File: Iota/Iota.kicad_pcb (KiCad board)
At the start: 2 copper layers, 22.6 x 43.4 mm, 23 parts, among them J1 USB_B_Mini, J2 Conn_01x12_Male, J3 Conn_01x12_Male, J4 Conn_01x05_Male, SW1 SW_DIP_x01, U1 ATmega32U4-MU, Y1 16MHz

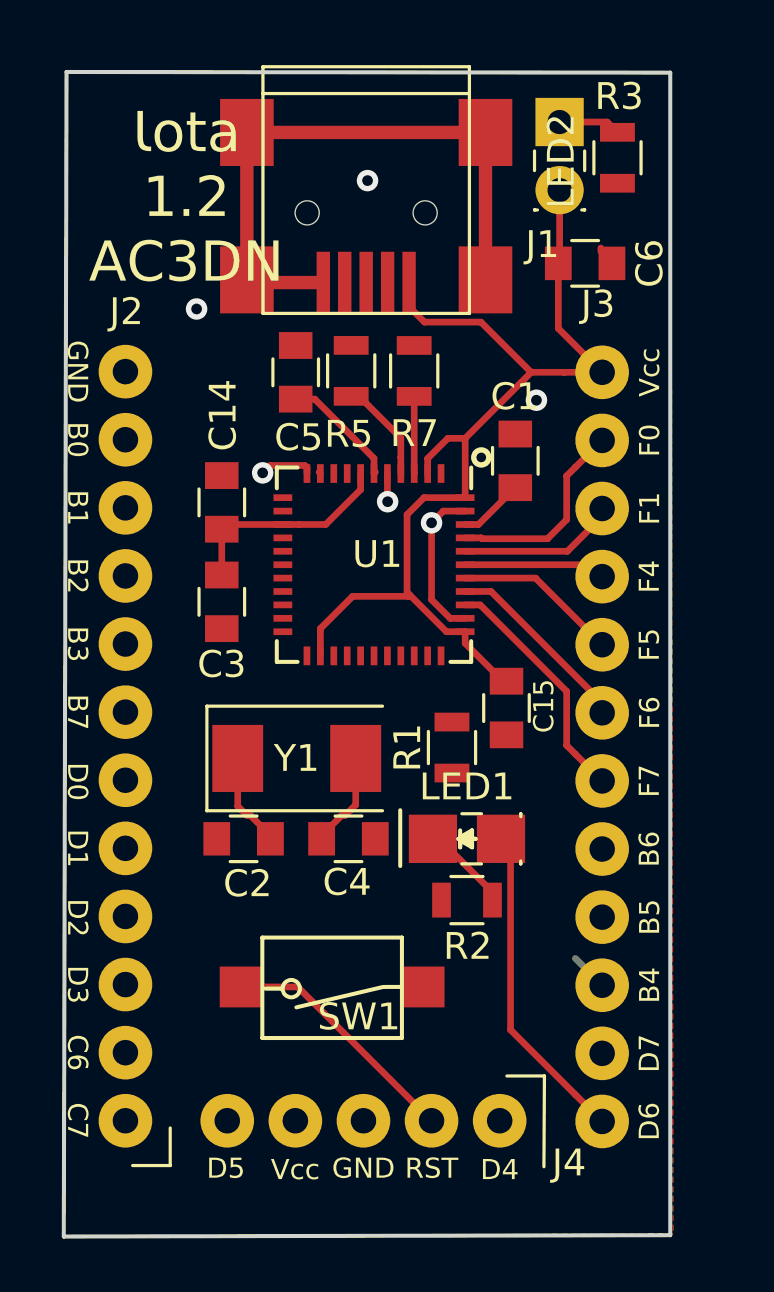
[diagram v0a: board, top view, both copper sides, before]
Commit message: Board layout is clean
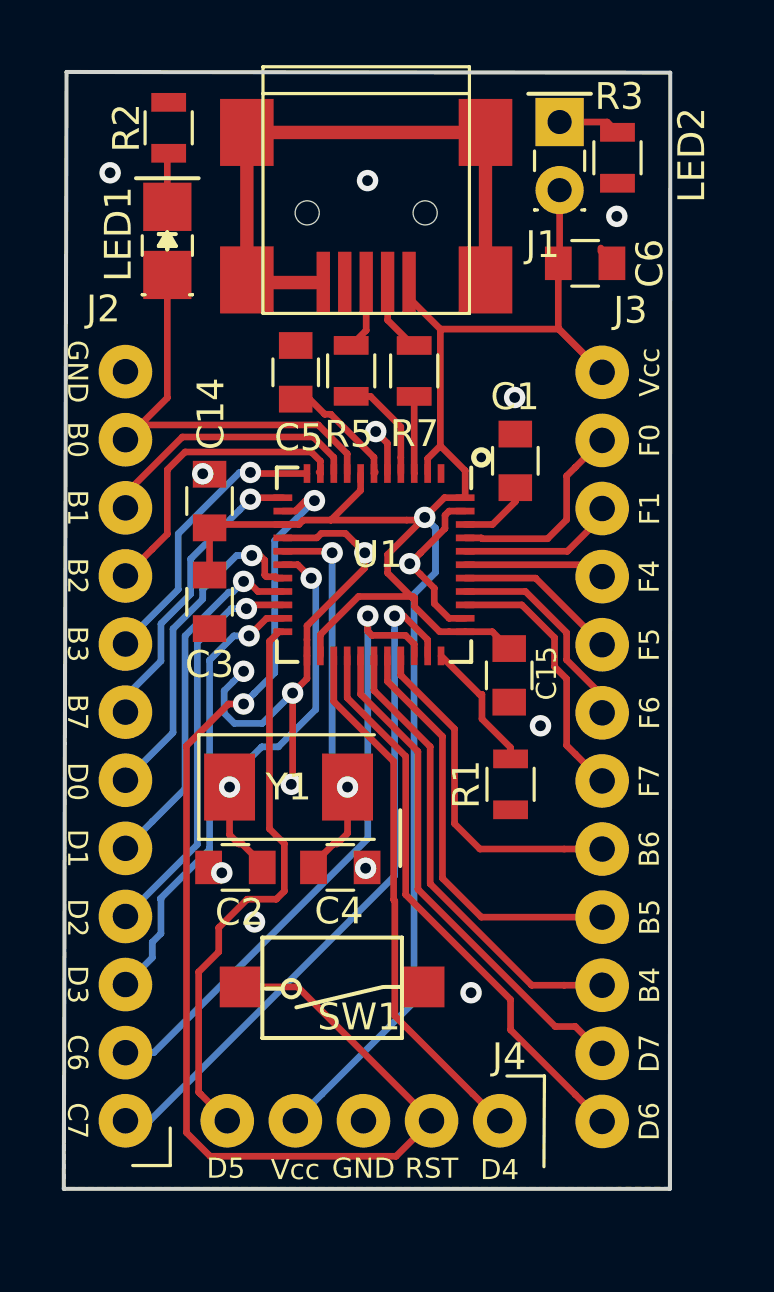
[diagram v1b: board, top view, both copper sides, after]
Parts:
- moved R2 30.9 mm to (126.1, 61.9), turned to 90 degrees
- moved G1 29.5 mm to (134.2, 93.5)
- moved LED1 25.6 mm to (126.1, 64.8), turned to 270 degrees
- moved R1 2.58 mm to (138.9, 86.4)
- moved C15 1.22 mm to (138.8, 82.3)
- moved C2 1.11 mm to (128.6, 89.5)
- moved C4 1.11 mm to (132.5, 89.5)
- moved Y1 1.11 mm to (130.6, 86.5)
- moved C14 0.46 mm to (127.7, 75.8)
- moved C3 0.46 mm to (127.7, 79.6)
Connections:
- LED1 pad 2: D6 -> B0
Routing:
- net RESET: track 9.20 -> 46.5 mm, vias 0 -> 2
- net Vcc: track 48.2 -> 76.6 mm, vias 0 -> 2
- net C7: track 0.00 -> 25.7 mm, vias 0 -> 1
- net C6: track 0.00 -> 23.6 mm, vias 0 -> 1
- net D5: track 0.00 -> 21.2 mm
- net D4: track 0.00 -> 19.9 mm
- net GND: track 29.8 -> 49.3 mm, vias 5 -> 16
- net D7: track 0.00 -> 19.0 mm
- net D3: track 0.00 -> 16.8 mm, vias 0 -> 1
- net B0: track 0.00 -> 16.5 mm
- net B4: track 1.41 -> 17.3 mm
- net B5: track 0.00 -> 15.7 mm
- net D2: track 0.00 -> 15.1 mm, vias 0 -> 1
- net D1: track 0.00 -> 13.5 mm, vias 0 -> 1
- net B6: track 0.00 -> 13.0 mm
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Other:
- board size 22.6 x 43.4 mm -> 22.6 x 41.7 mm

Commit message: Ready for PCB fabrication
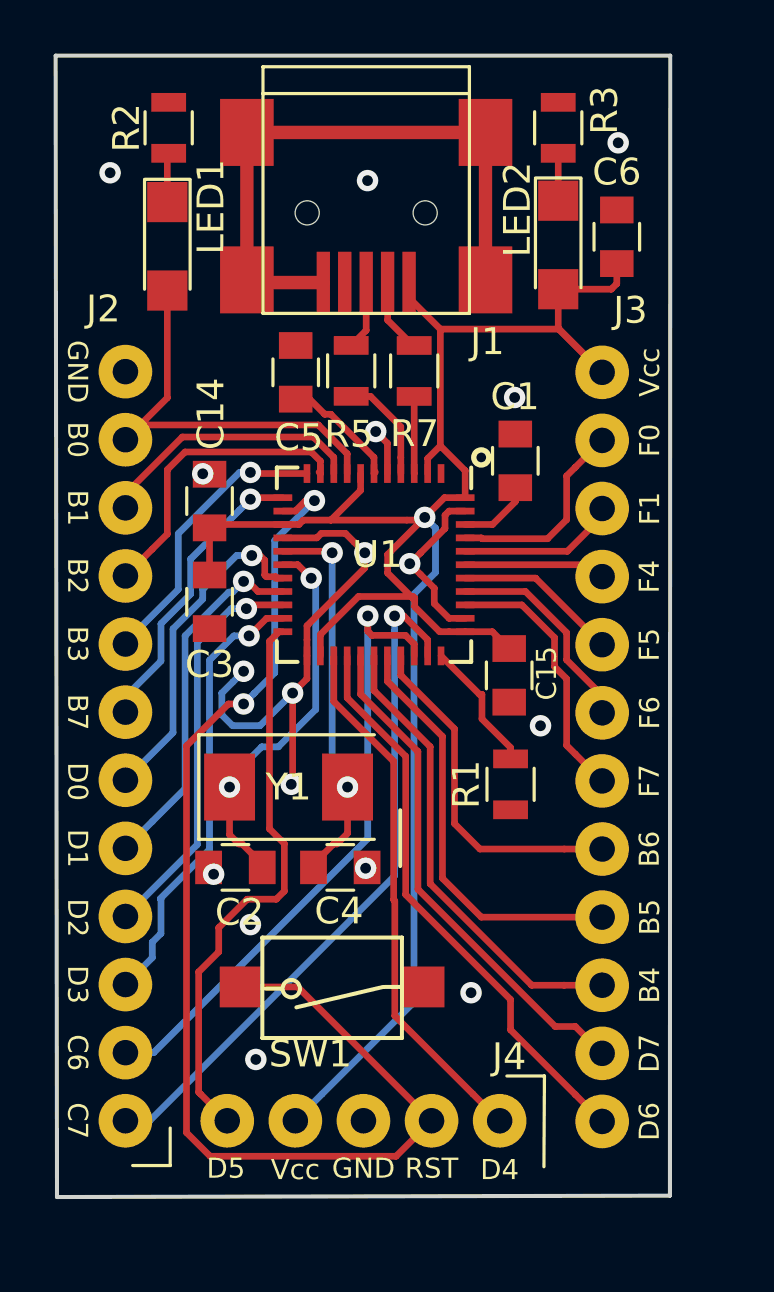
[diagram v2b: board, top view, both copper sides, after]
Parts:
- LED1, LED2: footprint LEDs:LED_Rectangular_W3.9mm_H1.8mm -> LEDs:LED_1206
- moved LED2 4.58 mm to (140.7, 66.2)
- moved R3 2.48 mm to (140.7, 61.9), turned to 90 degrees
- moved C6 1.54 mm to (142.8, 65.9), turned to 270 degrees
- moved LED1 1.47 mm to (126.1, 66.3)
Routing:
- net Vcc: track 76.6 -> 75.9 mm
- net B0: track 16.5 -> 15.9 mm
- net Net-(LED2-Pad1): track 2.32 -> 1.77 mm
- net GND: track 49.3 -> 49.4 mm, vias 16 -> 17
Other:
- board size 22.6 x 41.7 mm -> 22.9 x 42.6 mm
